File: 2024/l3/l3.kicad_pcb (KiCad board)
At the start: 2 copper layers, 137.5 x 129.1 mm, 23 parts, among them J1 Conn_01x04, SW1 SW_SPDT, SW2 SW_SPDT, SW3 SW_SPDT, SW4 SW_SPDT, U4 DEV-15583

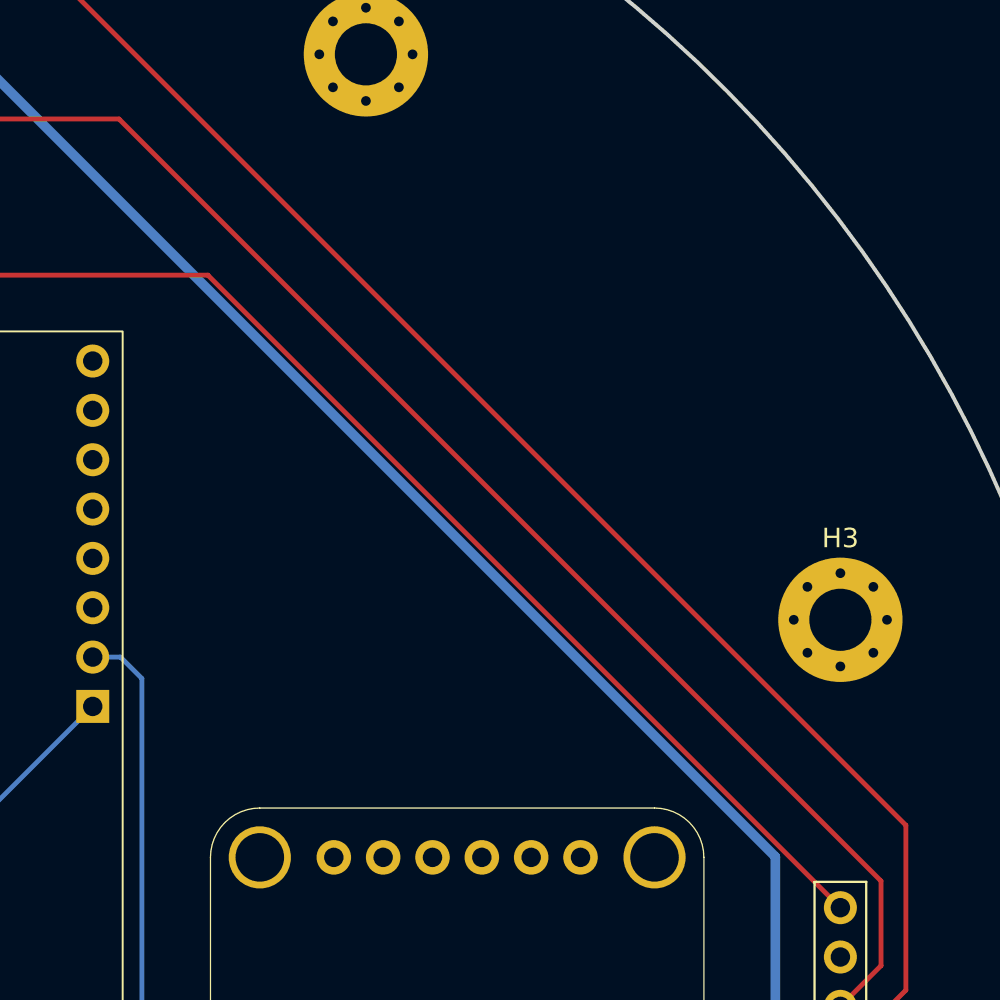
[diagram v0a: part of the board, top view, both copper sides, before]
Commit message: another test
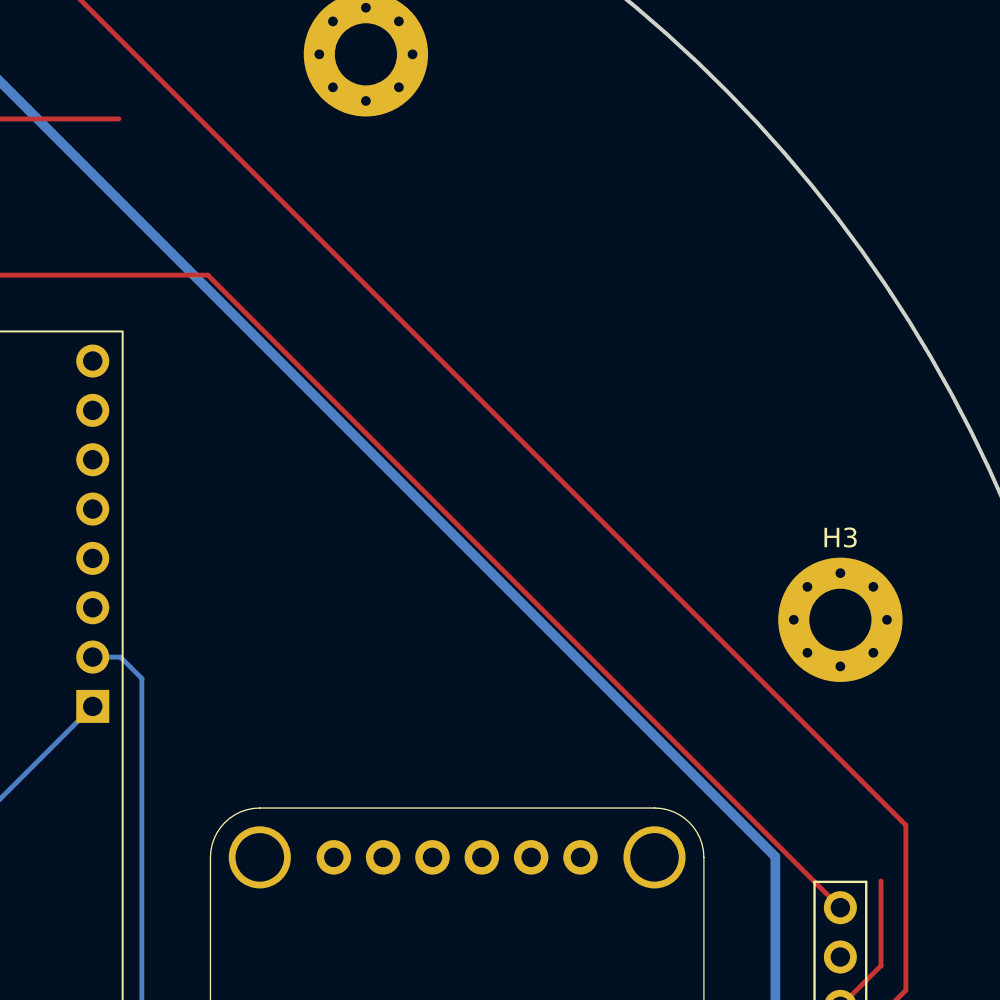
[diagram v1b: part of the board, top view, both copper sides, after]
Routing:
- net /SDAToF: track 281.1 -> 225.6 mm
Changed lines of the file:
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@@
-	)
-	(segment
-		(start 161.82 88.93)
-		(end 122.59 49.7)
-		(width 0.25)
-		(layer "F.Cu")
-		(net 5)
 	)
 	(segment

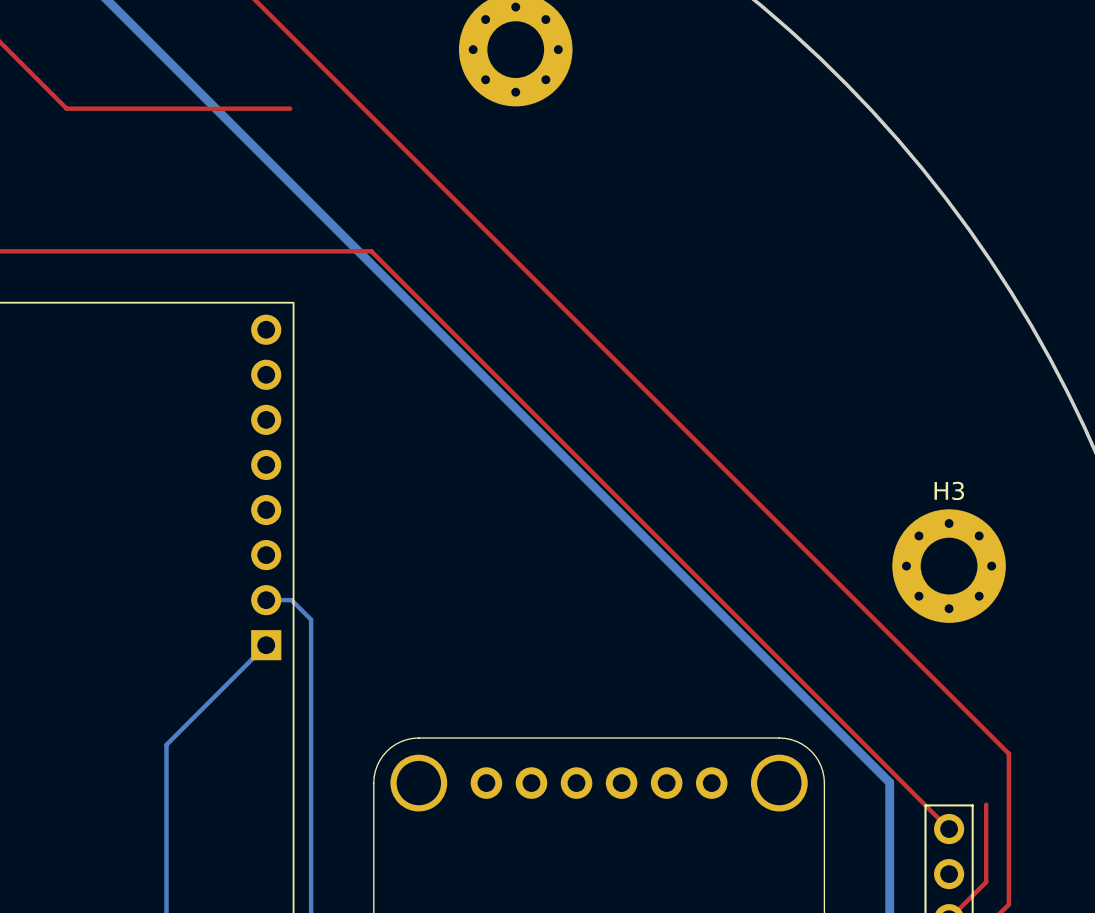
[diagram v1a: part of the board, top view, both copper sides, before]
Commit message: add back trace
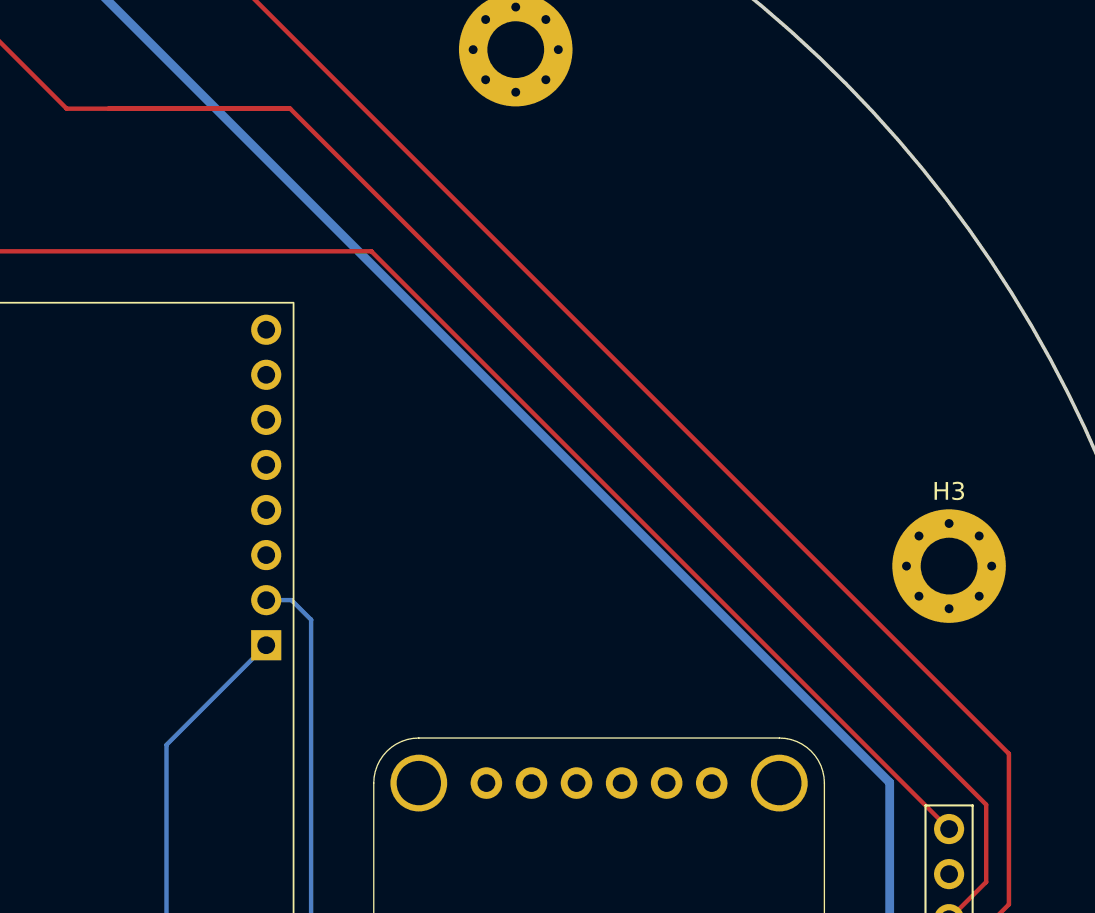
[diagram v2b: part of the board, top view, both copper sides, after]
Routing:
- net /SDAToF: track 225.6 -> 291.3 mm
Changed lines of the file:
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@@
+	)
+	(segment
+		(start 122.59 49.7)
+		(end 112.358751 49.7)
+		(width 0.25)
+		(layer "F.Cu")
+		(net 5)
 	)
 	(segment
@@
 		(width 0.25)
 		(layer "F.Cu")
+		(net 5)
+	)
+	(segment
+		(start 122.59 49.7)
+		(end 161.82 88.93)
+		(width 0.25)
+		(layer "F.Cu")
